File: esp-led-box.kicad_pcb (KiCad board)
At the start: 2 copper layers, 39 x 64 mm, 66 parts, among them IC1 CP2105-F01-GMR, J1 Conn_01x04, J2 Conn_01x02, J3 USB_B_Micro, J4 Conn_01x03_Female, J5 Conn_01x03_Female, Q1 2N7002, Q2 2N7002, Q3 Q_PMOS_DGS, Q4 Q_PMOS_DGS, Q5 S8050, Q6 S8050, Q7 Q_PMOS_DGS, Q8 2N7002, Q9 Q_PMOS_DGS, U1 LM3940, U2 MP2307, U3 ESP-12F, U4 LM211

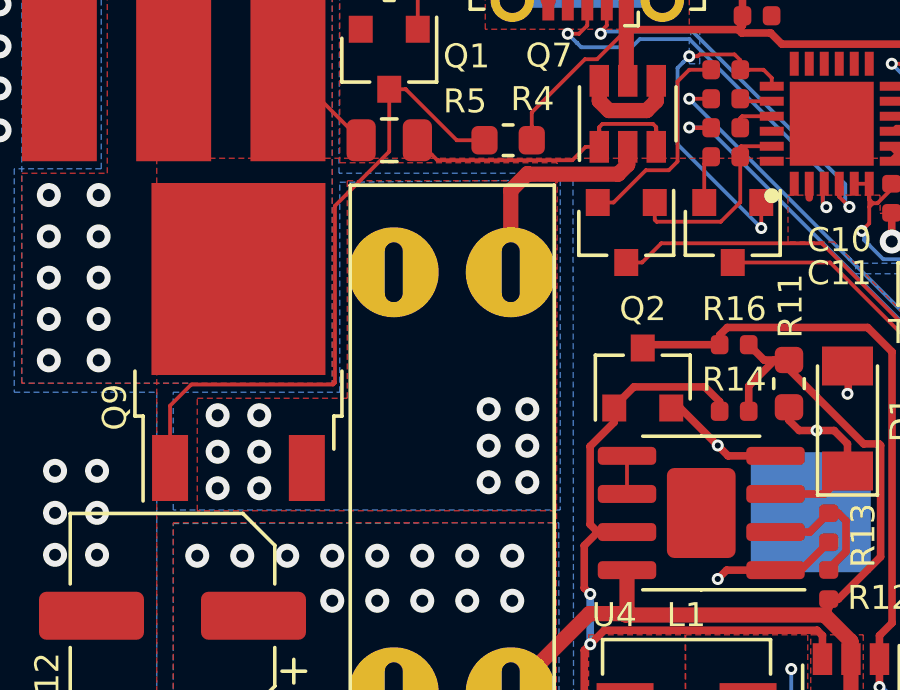
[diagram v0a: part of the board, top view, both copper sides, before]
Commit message: ~_~
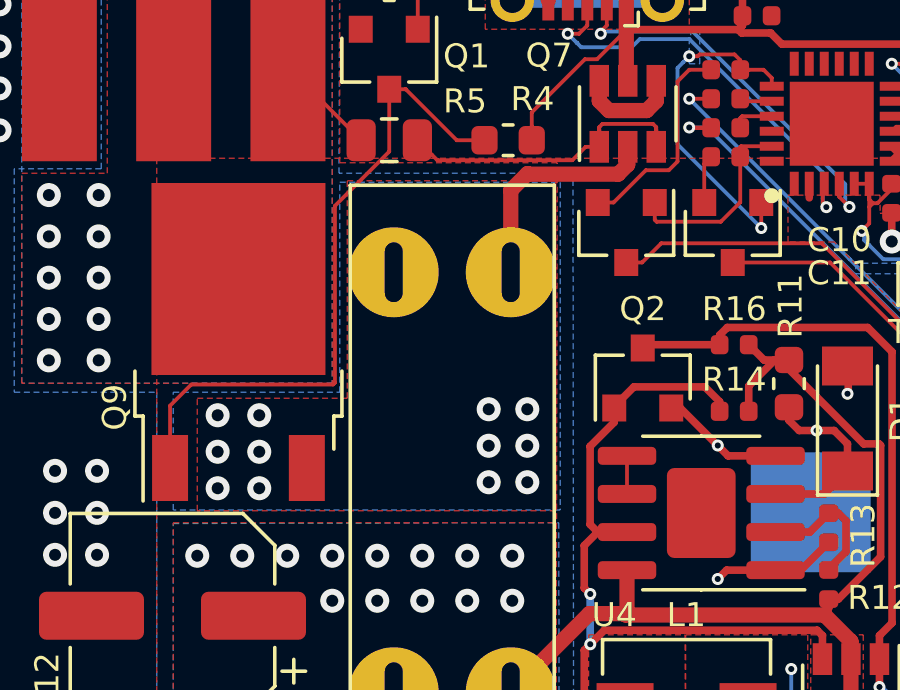
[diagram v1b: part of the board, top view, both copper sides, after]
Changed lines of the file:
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@@
       (pts
         (xy 75.85 71.225) (xy 62.95 71.225001) (xy 62.95 67.300002) (xy 68.5 67.3) (xy 68.5 60.3)
-        (xy 75.85 60.225)
+        (xy 75.85 60.3)
       )
     )
